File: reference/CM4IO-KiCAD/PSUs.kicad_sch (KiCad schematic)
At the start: 33 parts, among them J19 Barrel_Jack, J20 AMP171826-4, Q1 DMP3013SFV-7, U16 AP64501SP-13

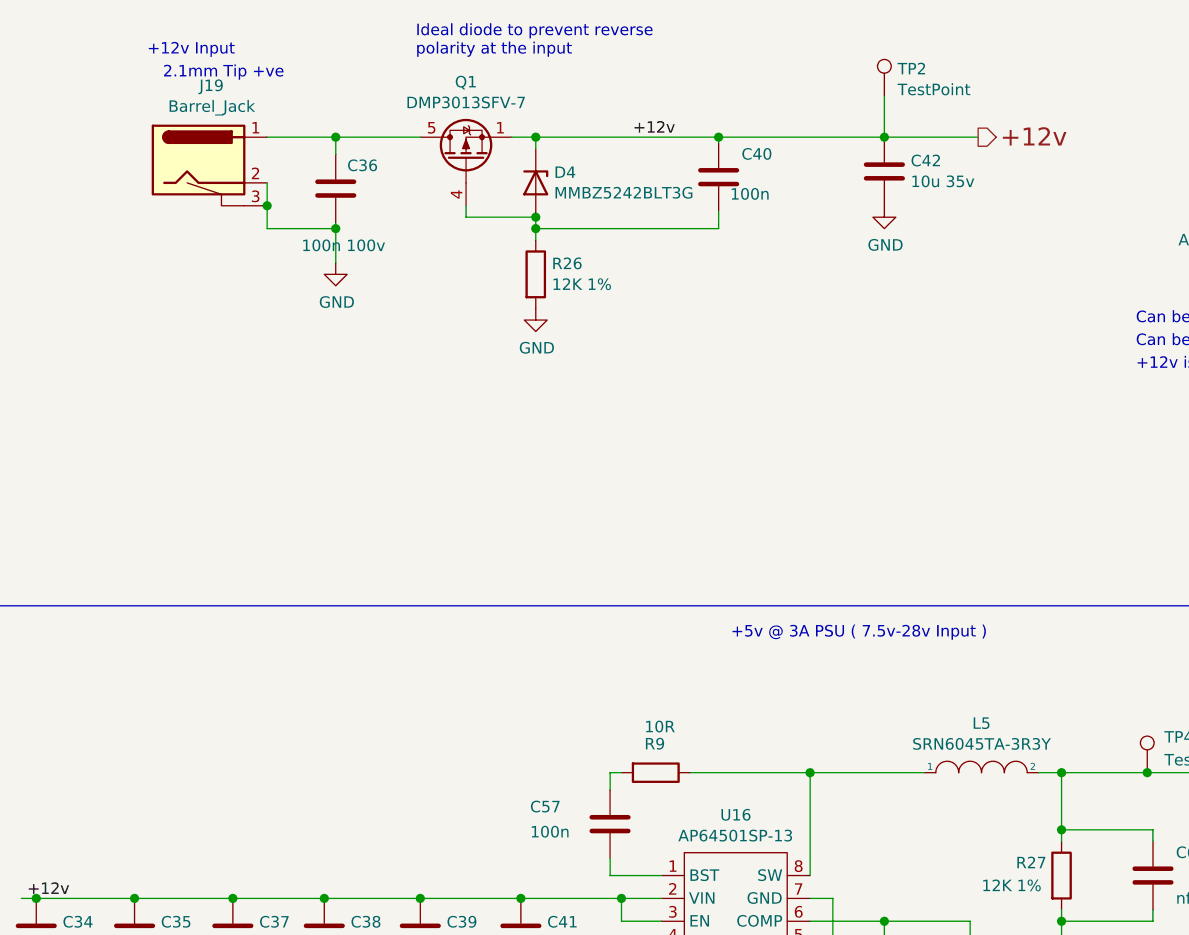
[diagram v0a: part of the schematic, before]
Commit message: Schaltplan Update
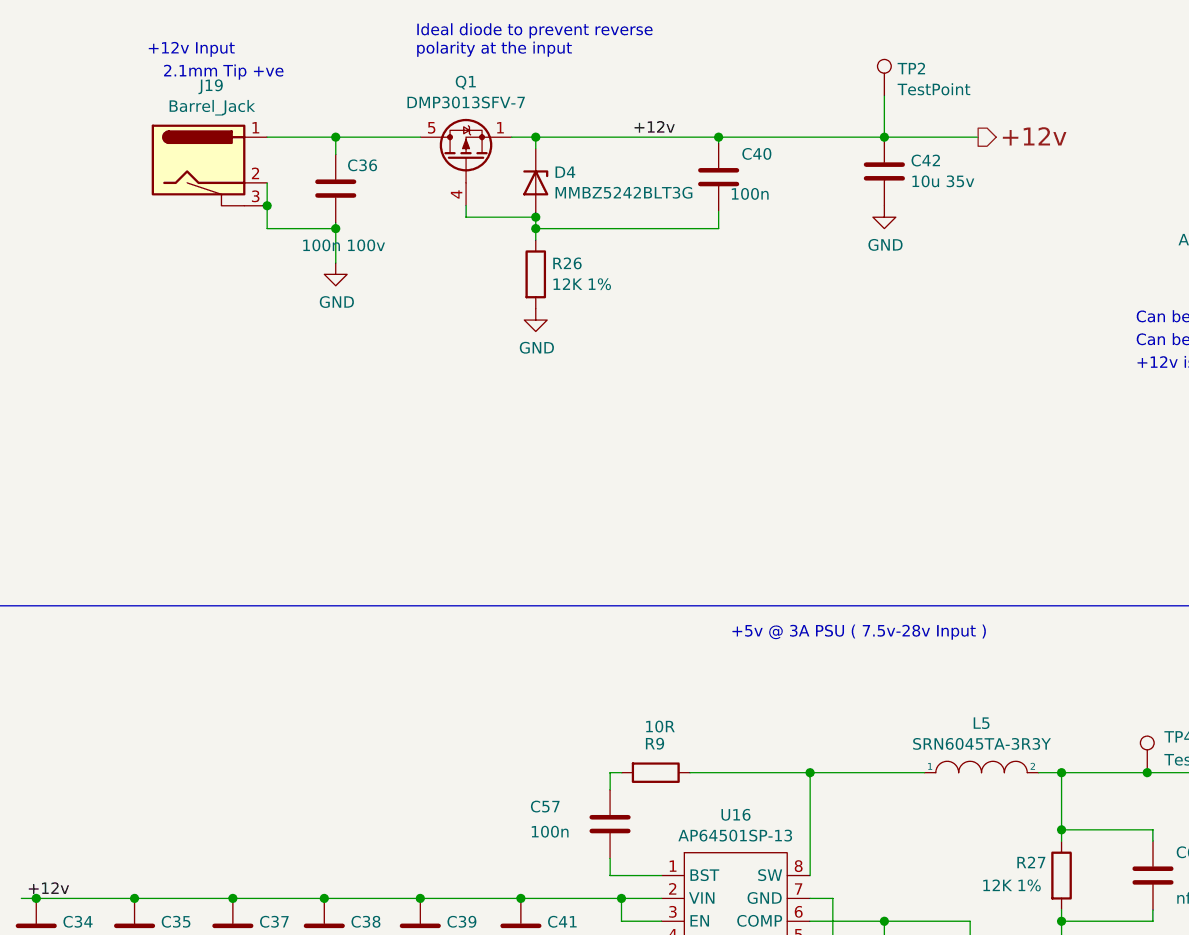
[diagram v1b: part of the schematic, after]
